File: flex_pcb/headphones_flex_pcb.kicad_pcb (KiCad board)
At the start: 2 copper layers, 41.7 x 25.7 mm, 34 parts, among them J1 LIGHTING_JACK, J2 CONN_01X01, J3 BOTTOM_FLEX_LIGHTNING, J5 LIGHTNING_HEADPHONE_ADAPTER, J7 IPHONE_HEADPHONE_JACK, U1 SN74LVC1G123, U2 SN74LVC1G123, U3 NC7S32-micropak6, U4 TS3Y5018RSV-UQFN

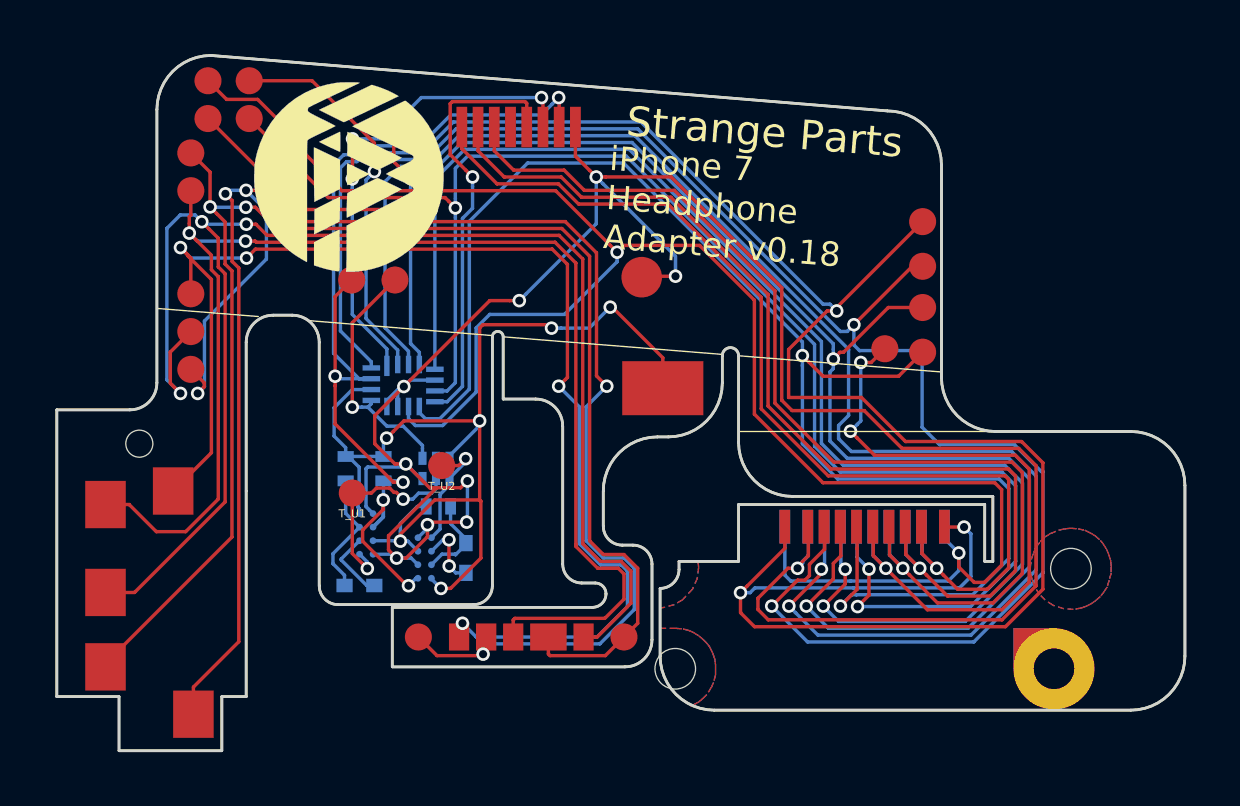
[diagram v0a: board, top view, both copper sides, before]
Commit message: Zigzag attempt 1
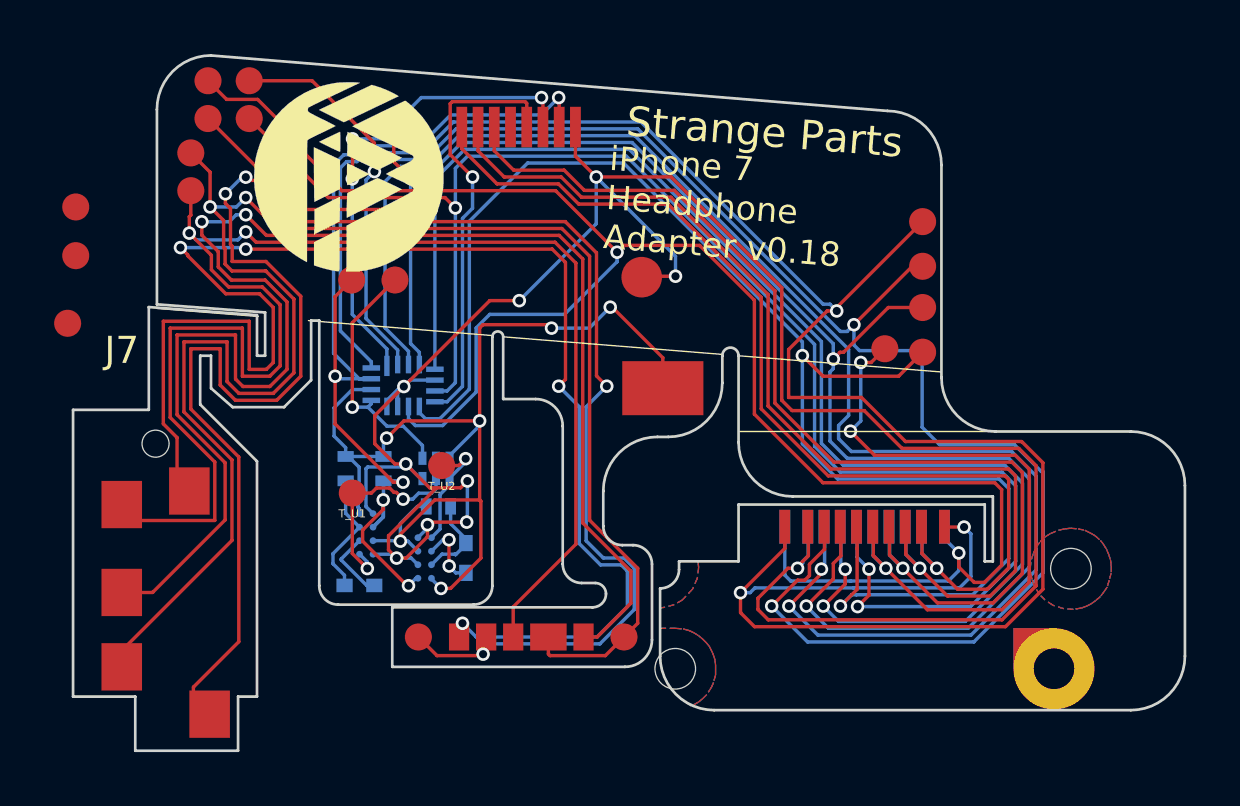
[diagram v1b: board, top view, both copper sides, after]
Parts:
- moved T_T2 5.33 mm to (123.5, 66.4)
- moved T_R1 5.10 mm to (123.5, 68.2)
- moved T_S1 4.86 mm to (123.2, 70.7)
- moved J7 0.60 mm to (125.2, 83.4)
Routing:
- net Net-(J5-Pad12): track 55.5 -> 65.0 mm
- net Net-(J5-Pad15): track 48.4 -> 55.0 mm
- net Net-(J5-Pad13): track 50.3 -> 56.5 mm
- net Net-(J5-Pad11): track 58.0 -> 57.3 mm, vias 3 -> 2
- net Net-(J5-Pad14): track 69.6 -> 69.4 mm, vias 5 -> 4
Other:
- board size 41.7 x 25.7 mm -> 41.1 x 25.7 mm
